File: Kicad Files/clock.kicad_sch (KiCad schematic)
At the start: 28 parts, among them SW1 SW_Push, SW2 SW_SPDT, U4 NE555P, U5 NE555P, U6 74HC04, U7 74HC00, U8 NE555P

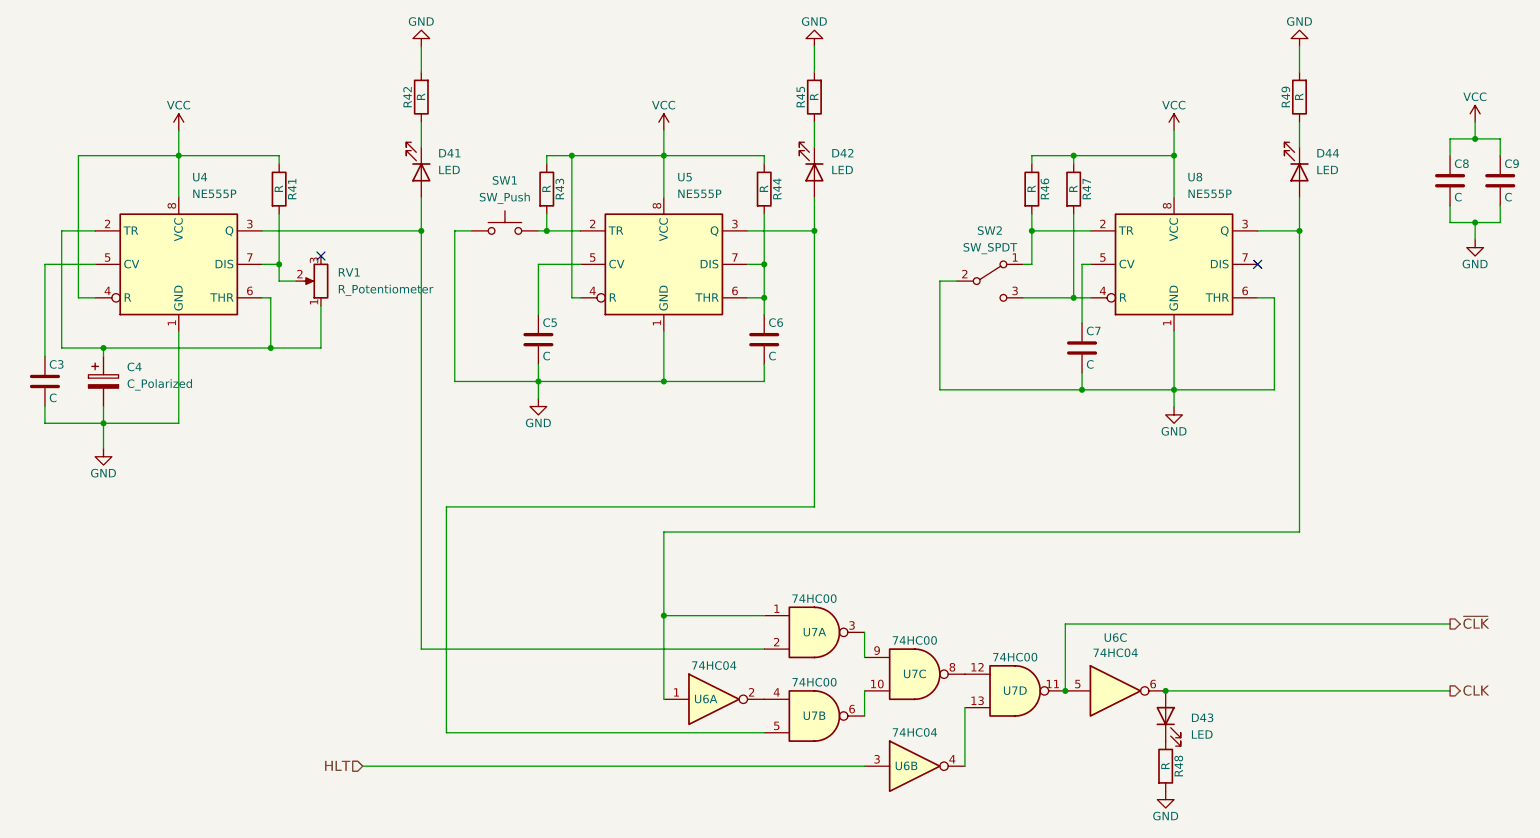
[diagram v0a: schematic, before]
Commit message: work on clk
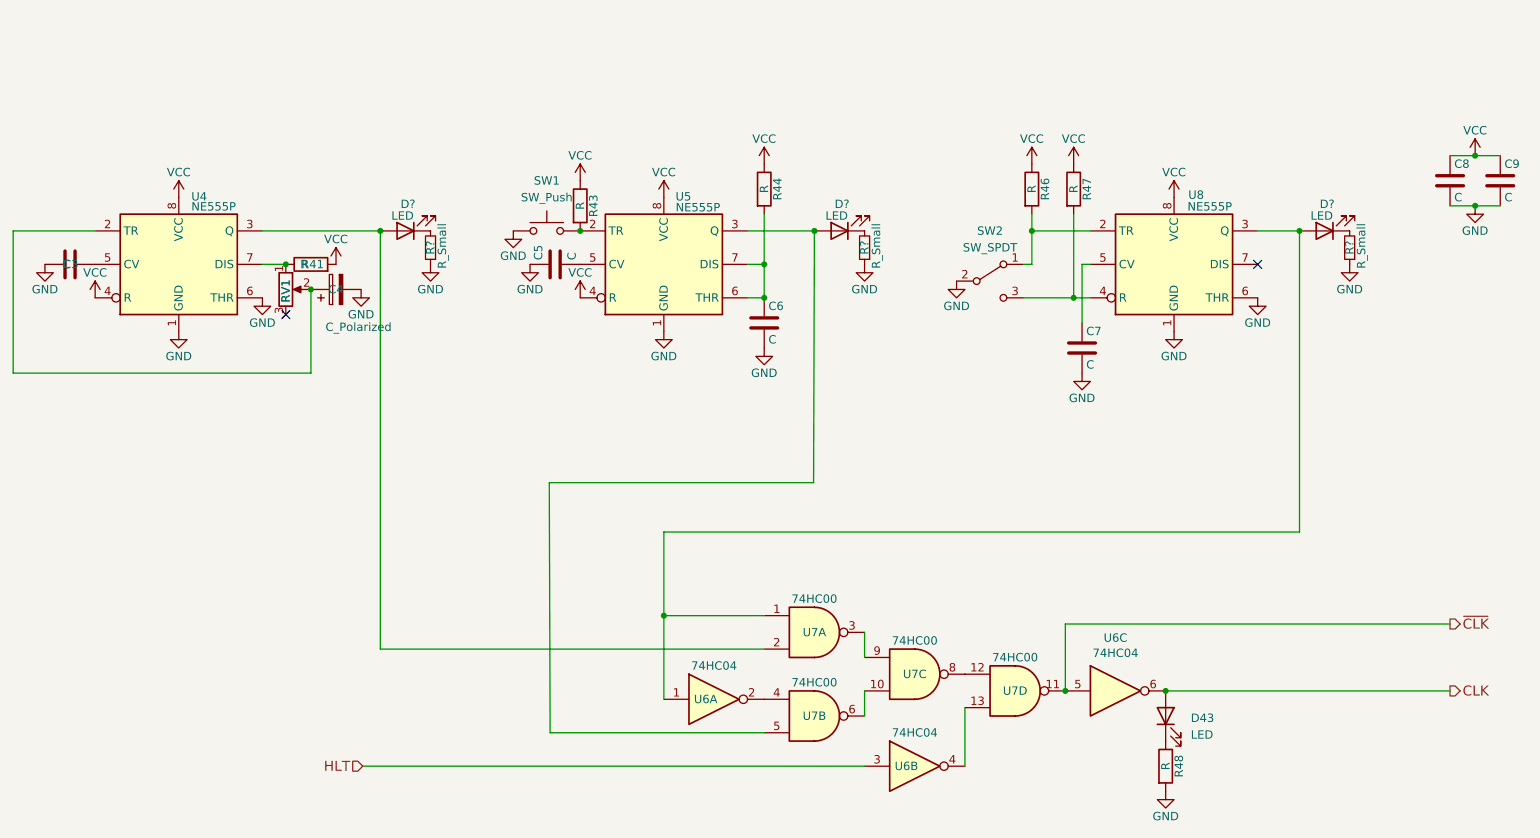
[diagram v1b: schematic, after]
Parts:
- removed D41, D42, D44: LED, symbol Device:LED
- removed R42, R45, R49: R, Resistor_THT:R_Axial_DIN0207_L6.3mm_D2.5mm_P7.62mm_Horizontal, symbol Device:R
- added D? (x3): LED, symbol Device:LED
- added R? (x3): R_Small, symbol Device:R_Small
- RV1: value R_Potentiometer -> RV1
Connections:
- net GND: now also C3.1, C5.1, U4.6 (THR), R?.1, R?.1, R?.1; no longer C3.2, C5.2
- net VCC: now also R41.2; no longer R41.1
- net at U4.5 (CV): now also C3.2; no longer C3.1
- net at U5.5 (CV): now also C5.2; no longer C5.1
- net at U6.1, U7.1, U8.3 (Q): now also D?.2 (A)
- net at U4.3 (Q), U7.2: now also D?.2 (A)
- net at U5.3 (Q), U7.5: now also D?.2 (A)
- net at C4.1, U4.2 (TR): now also RV1.2; no longer RV1.1, U4.6 (THR)
- new net: R41.1, RV1.1, U4.7 (DIS)
- new net: D?.1 (K), R?.2 (x3)
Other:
- moved on the sheet: C3, C4, C5, C6, R41, R43, RV1, SW1
